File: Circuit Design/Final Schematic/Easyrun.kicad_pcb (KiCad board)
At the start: 2 copper layers, 100 x 100 mm, 75 parts, among them U1 ESP32-WROOM-32

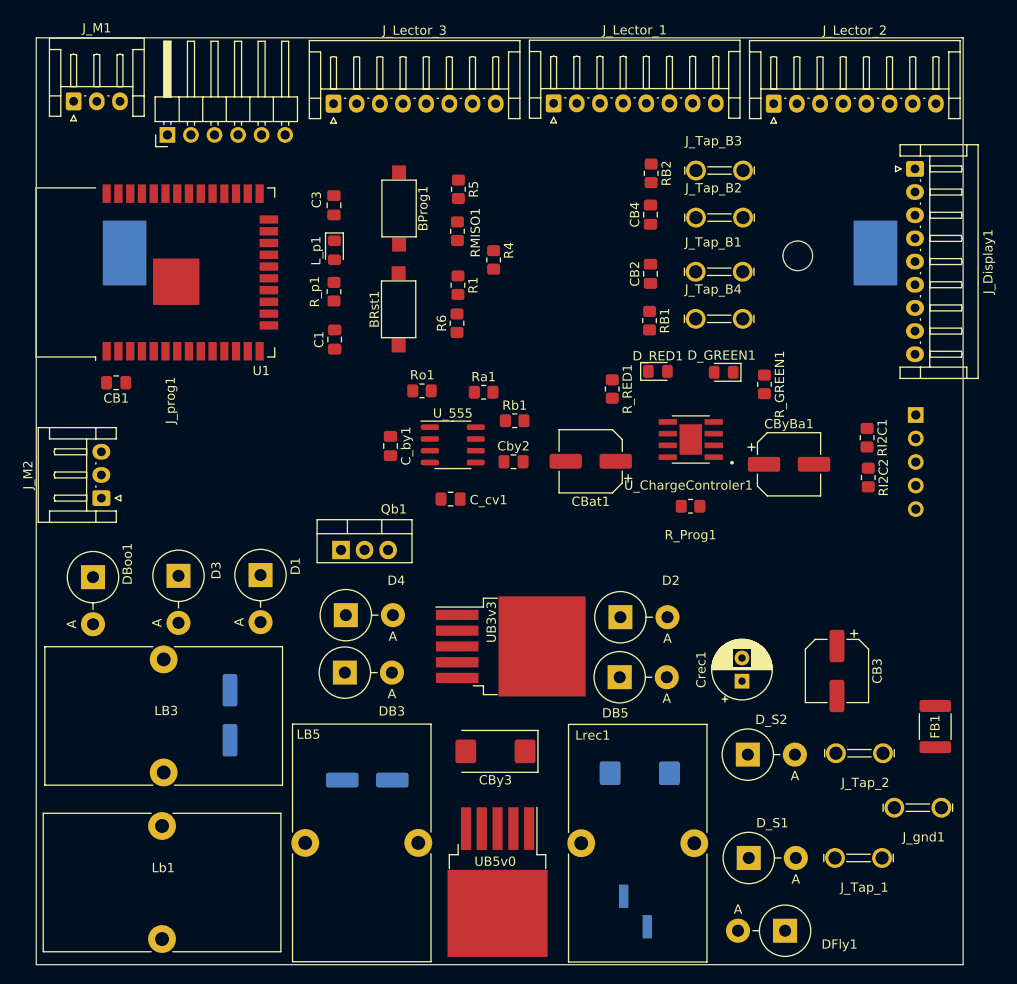
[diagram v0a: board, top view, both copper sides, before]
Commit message: More free space schematic
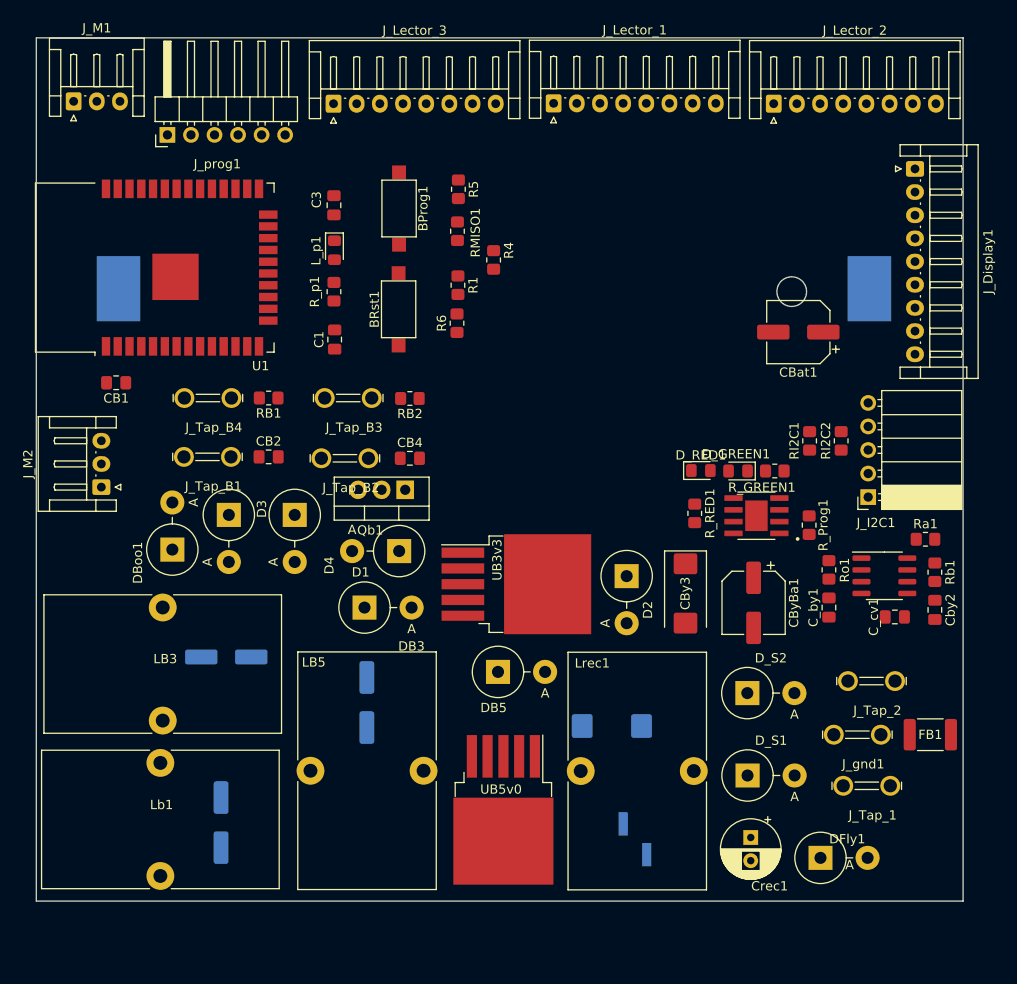
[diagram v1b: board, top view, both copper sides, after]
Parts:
- CB3: moved to B.Cu
- J_I2C1: moved to F.Cu
- moved CB3 65.9 mm to (92.5, 107.2), turned to 0 degrees
- moved J_Tap_B1 58.7 mm to (90.4, 85.6), turned to 180 degrees
- moved J_Tap_B4 55.8 mm to (90.5, 79.2), turned to 180 degrees
- moved C_by1 50.4 mm to (157.5, 101.9), turned to 90 degrees
- moved Ra1 50.2 mm to (167.9, 94.5)
- moved C_cv1 49.6 mm to (164.6, 102.9)
- moved U_555 48.7 mm to (163.5, 98.4)
- moved Rb1 48.2 mm to (168.9, 98.0), turned to -90 degrees
- moved Cby2 48.2 mm to (168.9, 102.1), turned to -90 degrees
- moved J_Tap_B2 48.0 mm to (105.3, 85.8), turned to 180 degrees
- moved Ro1 48.0 mm to (157.5, 97.8), turned to 90 degrees
- moved J_Tap_B3 47.0 mm to (105.6, 79.2), turned to 180 degrees
- moved CB2 45.7 mm to (97.0, 85.6), turned to 0 degrees
- moved RB1 41.9 mm to (97.0, 79.2), turned to 180 degrees
- moved CB4 36.9 mm to (112.3, 85.8), turned to 0 degrees
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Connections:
- D_RED1 pad 2: Net-(D_RED1-Pad2) -> /PowerModule/Buck5v0
- U1 pad 13: /CS_Lector3 -> CHRG
- U1 pad 14: unconnected-(U1-Pad14) -> STDBY
- U1 pad 24: unconnected-(U1-Pad24) -> /CS_Lector3
- U_ChargeControler1 pad 8: Net-(D_RED1-Pad2) -> /PowerModule/Buck5v0
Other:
- board size 100 x 100 mm -> 100 x 93.1 mm
